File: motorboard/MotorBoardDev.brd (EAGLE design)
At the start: 86 x 80.5 mm, 70 parts, among them J1 Under Glow, J2 B2PS-VH(LF)(SN), J3 B2PS-VH(LF)(SN), J4 B2PS-VH(LF)(SN), Q1 SSM3J338R, Q2 SSM3J338R, Q3 SSM3J338R, Q4 STT4P3LLH6, U1 TXB0104DR, U2 9DoF IMU, U3 TXB0106PWR, U4 TLV70233DBVR, X1 C-GRID-05-15-91, X2 C-GRID-05-15-91, X3 MINI-USB_SHIELD5P4-32005-400, X4 C-GRID-02-70553, X5 SI-50170, X7 2510-, X8 2510-

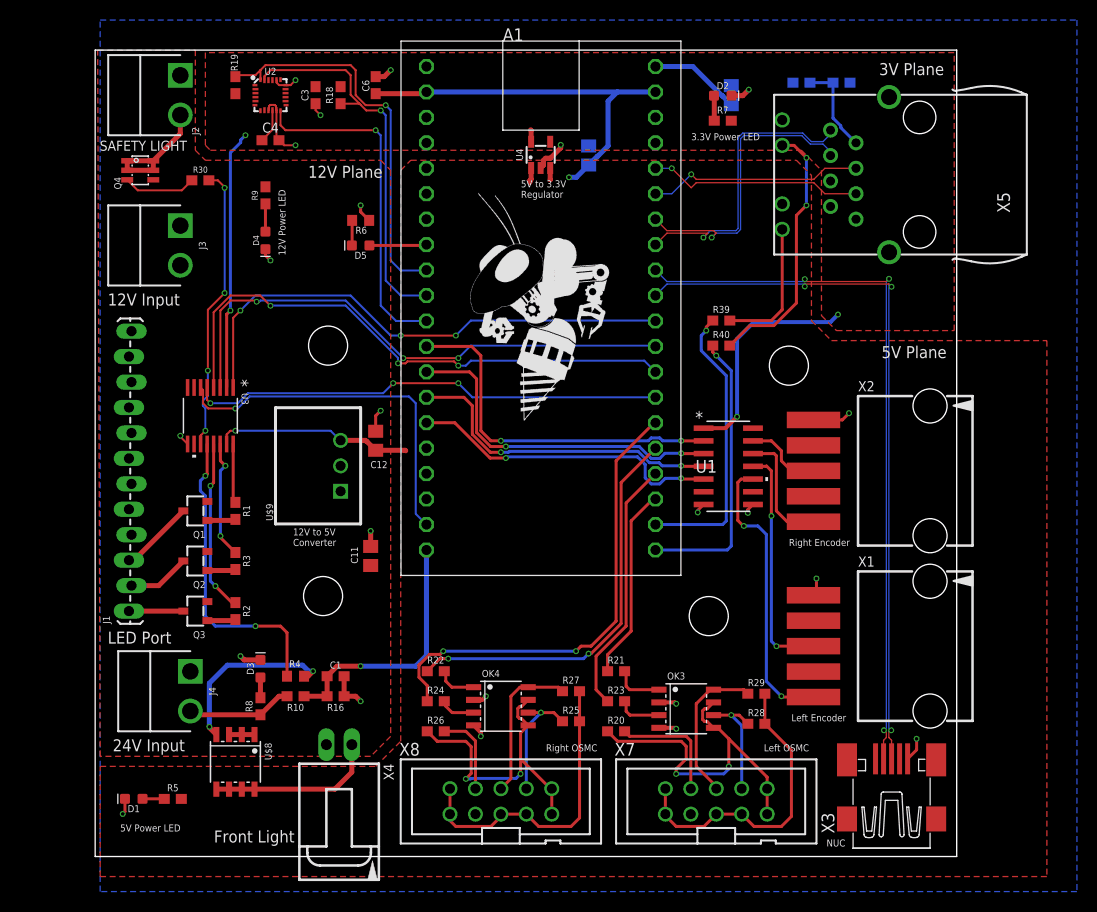
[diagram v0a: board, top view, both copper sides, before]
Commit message: moved board
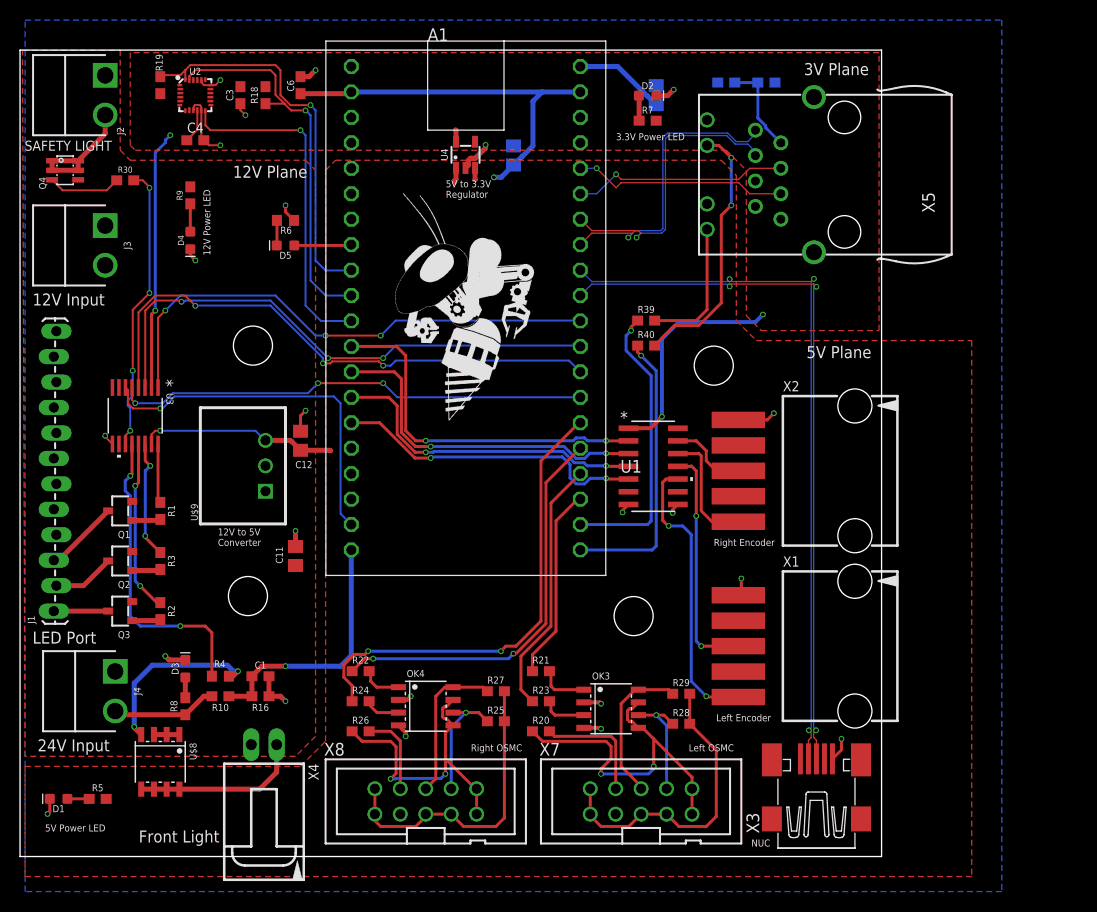
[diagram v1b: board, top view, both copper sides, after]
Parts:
- moved D2 7.50 mm to (62.6, 76.0)
- moved R7 7.50 mm to (62.6, 73.5)
- moved A1 7.50 mm to (44.5, 56.0)
- moved C1 7.50 mm to (24.0, 18.0)
- moved C11 7.50 mm to (27.5, 30.0)
- moved C12 7.50 mm to (28.0, 41.5)
- moved C13 7.50 mm to (49.3, 70.0)
- moved C14 7.50 mm to (63.5, 76.0)
- moved C2 7.50 mm to (74.5, 77.2)
- moved C3 7.50 mm to (22.0, 76.0)
- moved C4 7.50 mm to (17.5, 71.5)
- moved C5 7.50 mm to (70.5, 77.2)
- moved C6 7.50 mm to (28.0, 77.0)
- moved D1 7.50 mm to (3.85, 5.76)
- moved D3 7.50 mm to (16.5, 18.8)
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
